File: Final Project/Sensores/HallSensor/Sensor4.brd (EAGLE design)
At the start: 14.4 x 12.6 mm, 5 parts

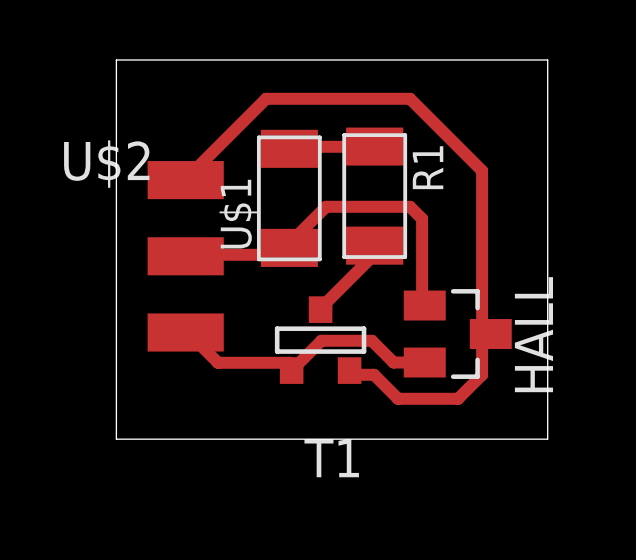
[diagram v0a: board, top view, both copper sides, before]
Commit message: sensor
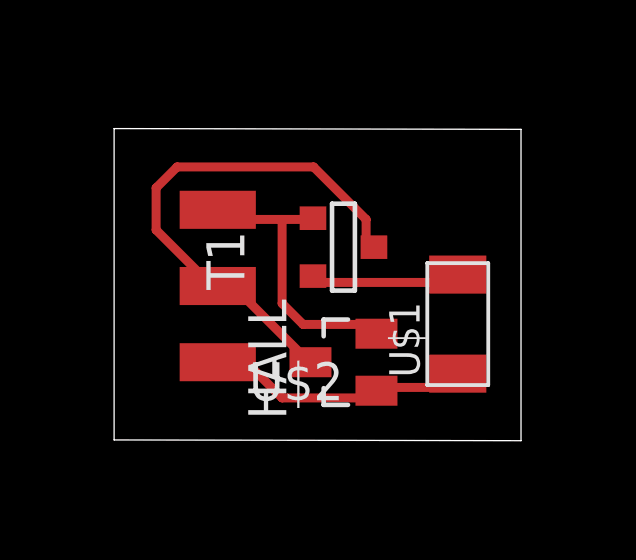
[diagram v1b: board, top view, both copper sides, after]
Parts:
- removed R1: (no value), fab:R1206FAB
- moved U$1 7.01 mm to (11.5, 3.86)
- moved HALL 3.92 mm to (7.65, 2.59), turned to 90 degrees
- moved T1 3.16 mm to (7.65, 6.40), turned to 90 degrees
- moved U$2 2.08 mm to (3.84, 5.13), turned to 180 degrees
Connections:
- removed net N$1: R1.1, U$1.2
- removed net N$2: R1.2, T1.1
- new net IN: T1.2, U$1.2
- net GND: now also T1.1, U$2.2; no longer T1.2, U$2.1
- net VCC: now also U$2.1; no longer U$2.2
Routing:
- net GND: track 24.3 -> 17.5 mm
- net IN: track 0.00 -> 5.13 mm
- net N$1: track 2.89 -> 0.00 mm
- net N$2: track 2.86 -> 0.00 mm
- net VCC: track 11.7 -> 8.89 mm
- net ANALOG: track 9.30 -> 9.81 mm
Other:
- board size 14.4 x 12.6 mm -> 13.6 x 10.4 mm
